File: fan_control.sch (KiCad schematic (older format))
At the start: 11 parts, among them M1 Fan, Q2 IRFZ34N, U1 LM317_3PinPackage

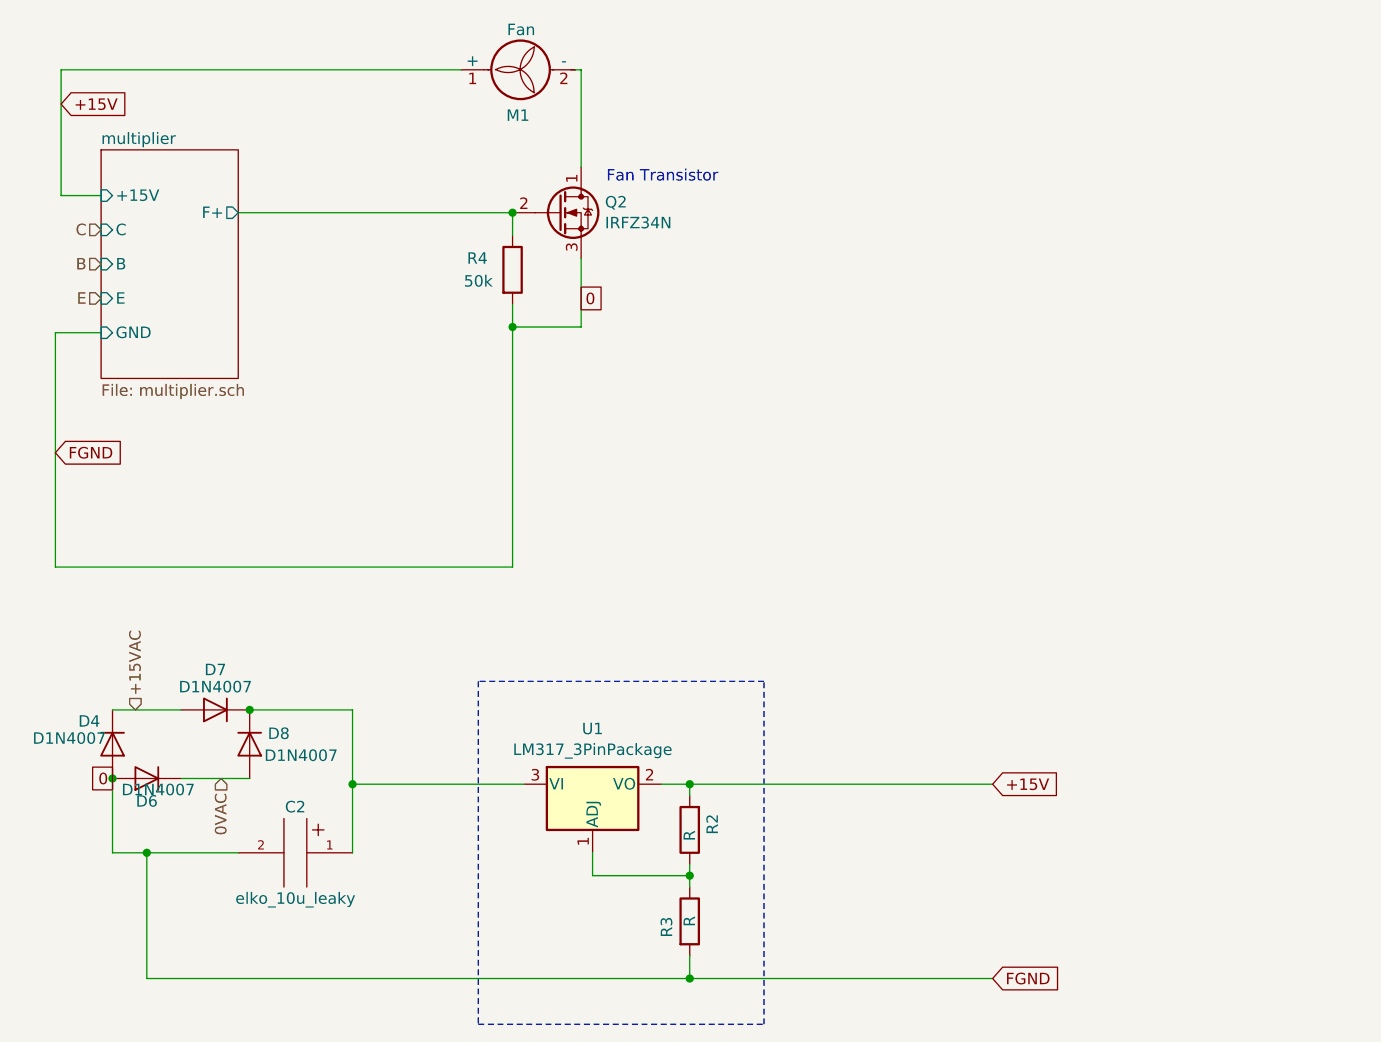
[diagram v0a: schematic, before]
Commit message: progress on schematics
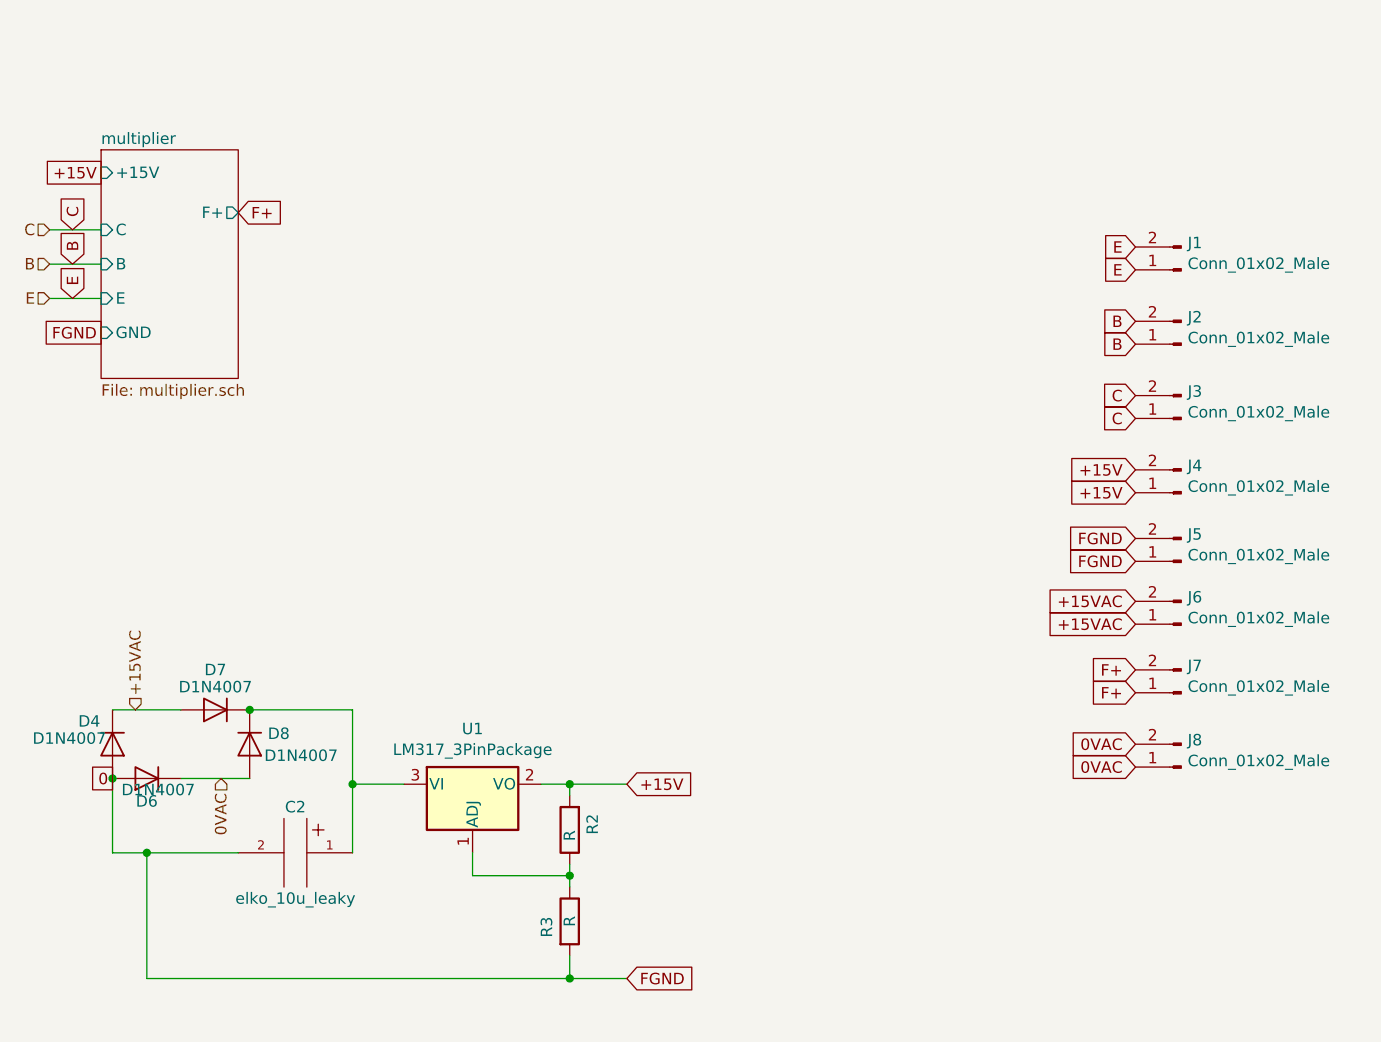
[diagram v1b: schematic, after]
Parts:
- removed M1: Fan, Connector_PinHeader_2.54mm:PinHeader_1x02_P2.54mm_Vertical, symbol Motor:Fan
- removed Q2: IRFZ34N, Package_TO_SOT_THT:TO-220-3_Vertical, symbol 0_project:IRFZ34N
- removed R4: 50k, Resistor_THT:R_Axial_DIN0207_L6.3mm_D2.5mm_P2.54mm_Vertical, symbol Device:R
- added J1, J2, J3, J4, J5, J6, J7, J8: Conn_01x02_Male, Connector_PinHeader_2.54mm:PinHeader_1x02_P2.54mm_Vertical, symbol Connector:Conn_01x02_Male
- D4: footprint (none) -> Diode_THT:D_DO-41_SOD81_P2.54mm_Vertical_AnodeUp
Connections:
- net +15V: now also J4.1 (Pin_1), J4.2 (Pin_2)
- net +15VAC: now also J6.1 (Pin_1), J6.2 (Pin_2)
- net 0: now also J5.1 (Pin_1), J5.2 (Pin_2)
- net 0VAC: now also J8.1 (Pin_1), J8.2 (Pin_2)
- net B: now also J2.1 (Pin_1), J2.2 (Pin_2)
- net C: now also J3.1 (Pin_1), J3.2 (Pin_2)
- net E: now also J1.1 (Pin_1), J1.2 (Pin_2)
- new net F+: J7.1 (Pin_1), J7.2 (Pin_2)
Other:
- note removed: "Fan Transistor"
- moved on the sheet: R2, R3, U1
